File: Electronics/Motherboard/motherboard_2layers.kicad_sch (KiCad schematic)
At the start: 55 parts, among them J1 DX07S024JJ3R1300, J2 Conn_02x10_Odd_Even, M1 AO3400A, M2 AO3400A, M3 AO3400A, U1 AMS1117-3.3, U2 TMC2209_SILENTSTEPSTICK, U3 TMC2209_SILENTSTEPSTICK, U4 TMC2209_SILENTSTEPSTICK, U5 TMC2209_SILENTSTEPSTICK, U6 LM2576HVS-5, U7 STM32G0B1VETx

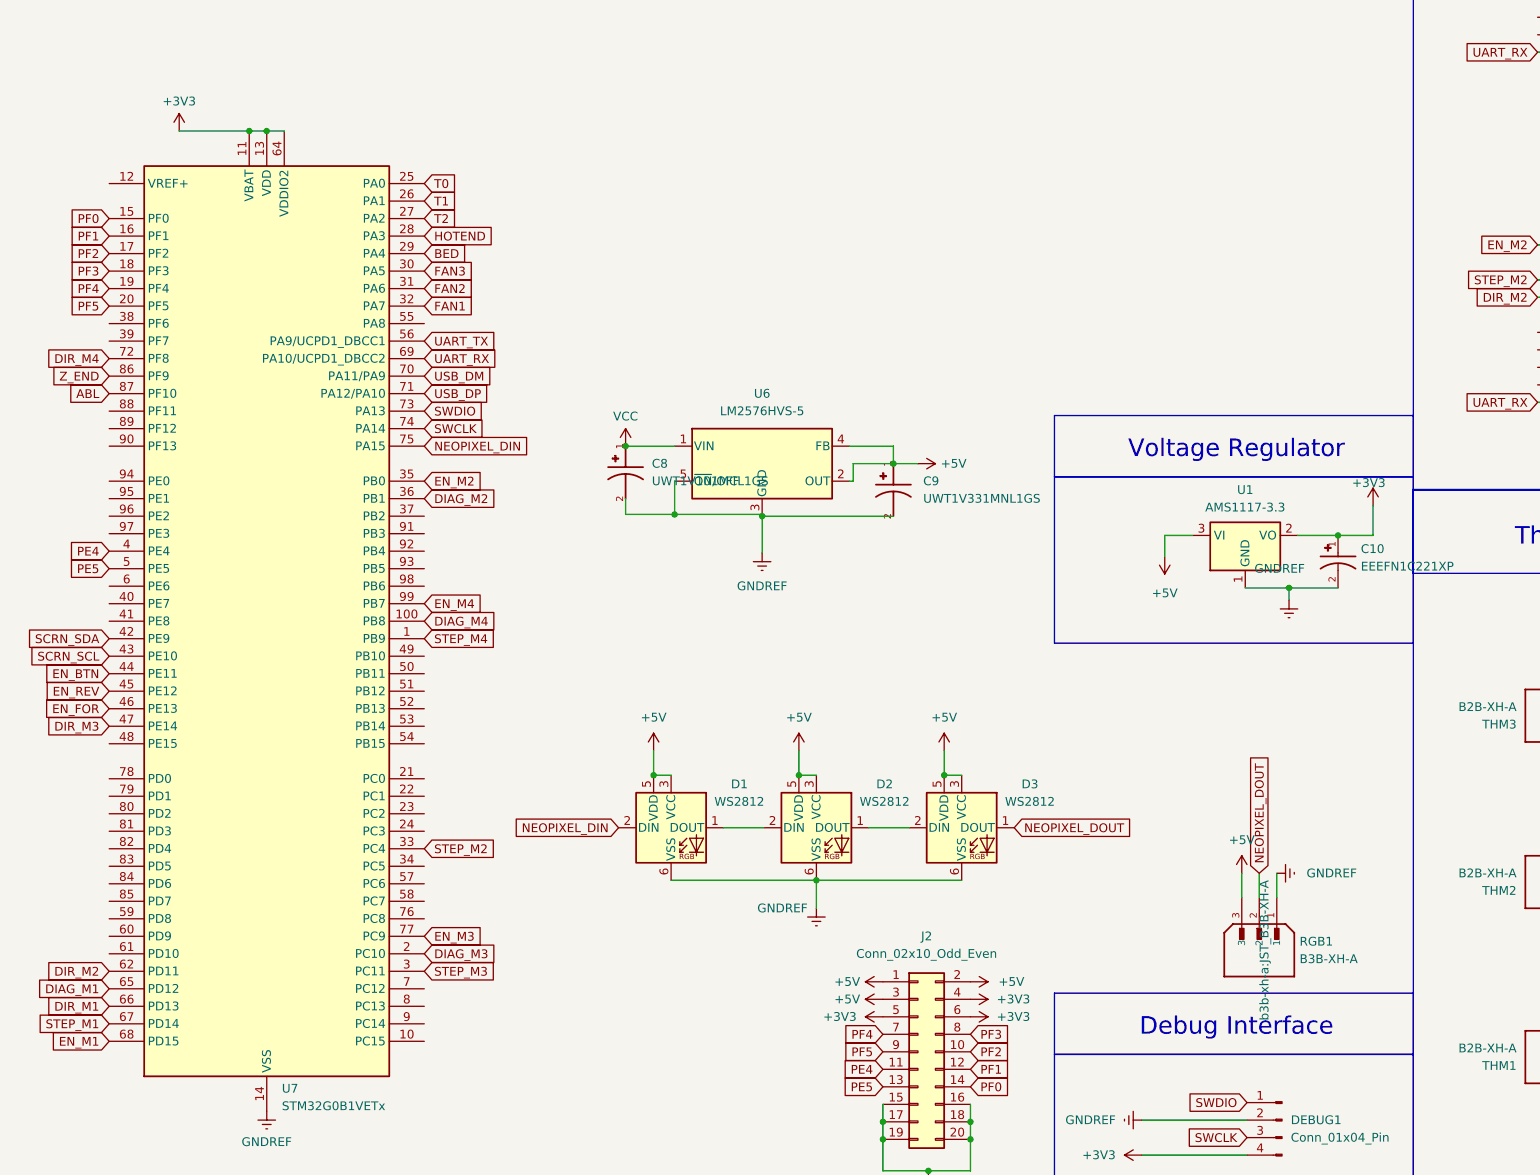
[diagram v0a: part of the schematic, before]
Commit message: yay finished
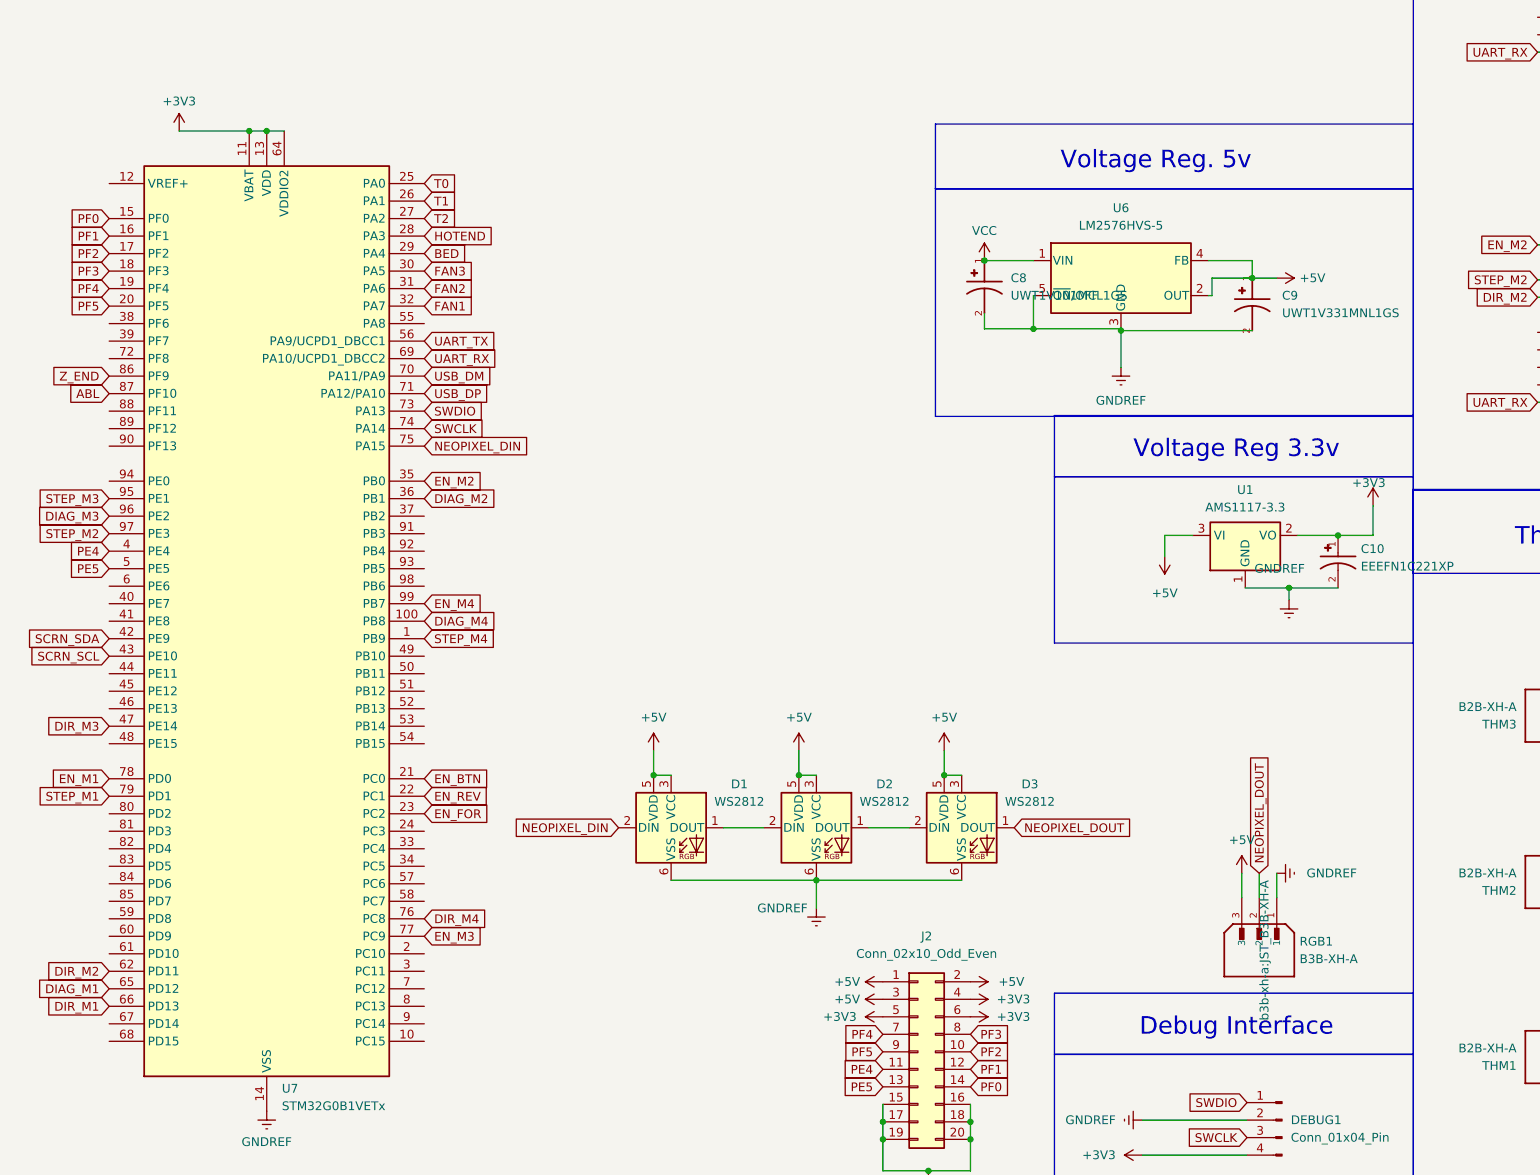
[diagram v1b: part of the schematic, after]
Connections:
- net DIAG_M3: now also U7.96 (PE2); no longer U7.2 (PC10)
- net DIR_M4: now also U7.76 (PC8); no longer U7.72 (PF8)
- net EN_BTN: now also U7.21 (PC0); no longer U7.44 (PE11)
- net EN_FOR: now also U7.23 (PC2); no longer U7.46 (PE13)
- net EN_M1: now also U7.78 (PD0); no longer U7.68 (PD15)
- net EN_REV: now also U7.22 (PC1); no longer U7.45 (PE12)
- net STEP_M1: now also U7.79 (PD1); no longer U7.67 (PD14)
- net STEP_M2: now also U7.97 (PE3); no longer U7.33 (PC4)
- net STEP_M3: now also U7.95 (PE1); no longer U7.3 (PC11)
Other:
- note added: "Voltage Reg 3.3v"
- note added: "Voltage Reg. 5v"
- note removed: "Voltage Regulator"
- moved on the sheet: C8, C9, U6

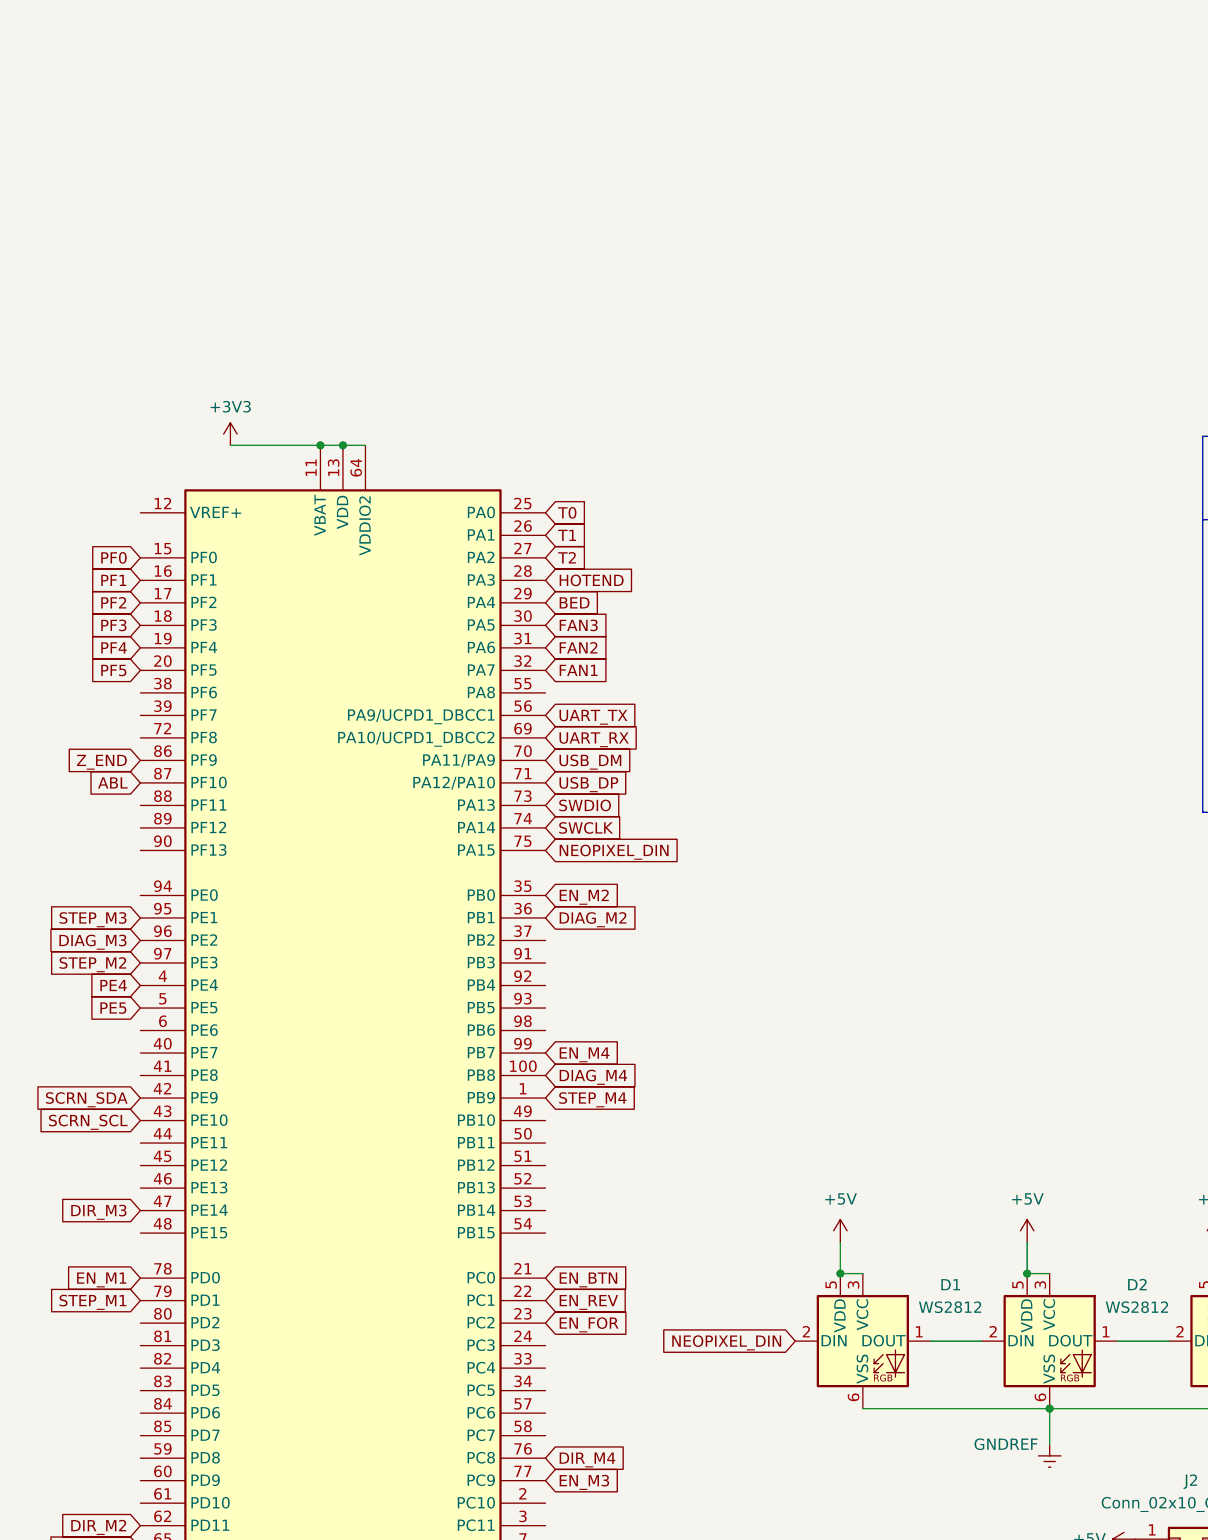
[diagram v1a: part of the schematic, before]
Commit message: updated some files
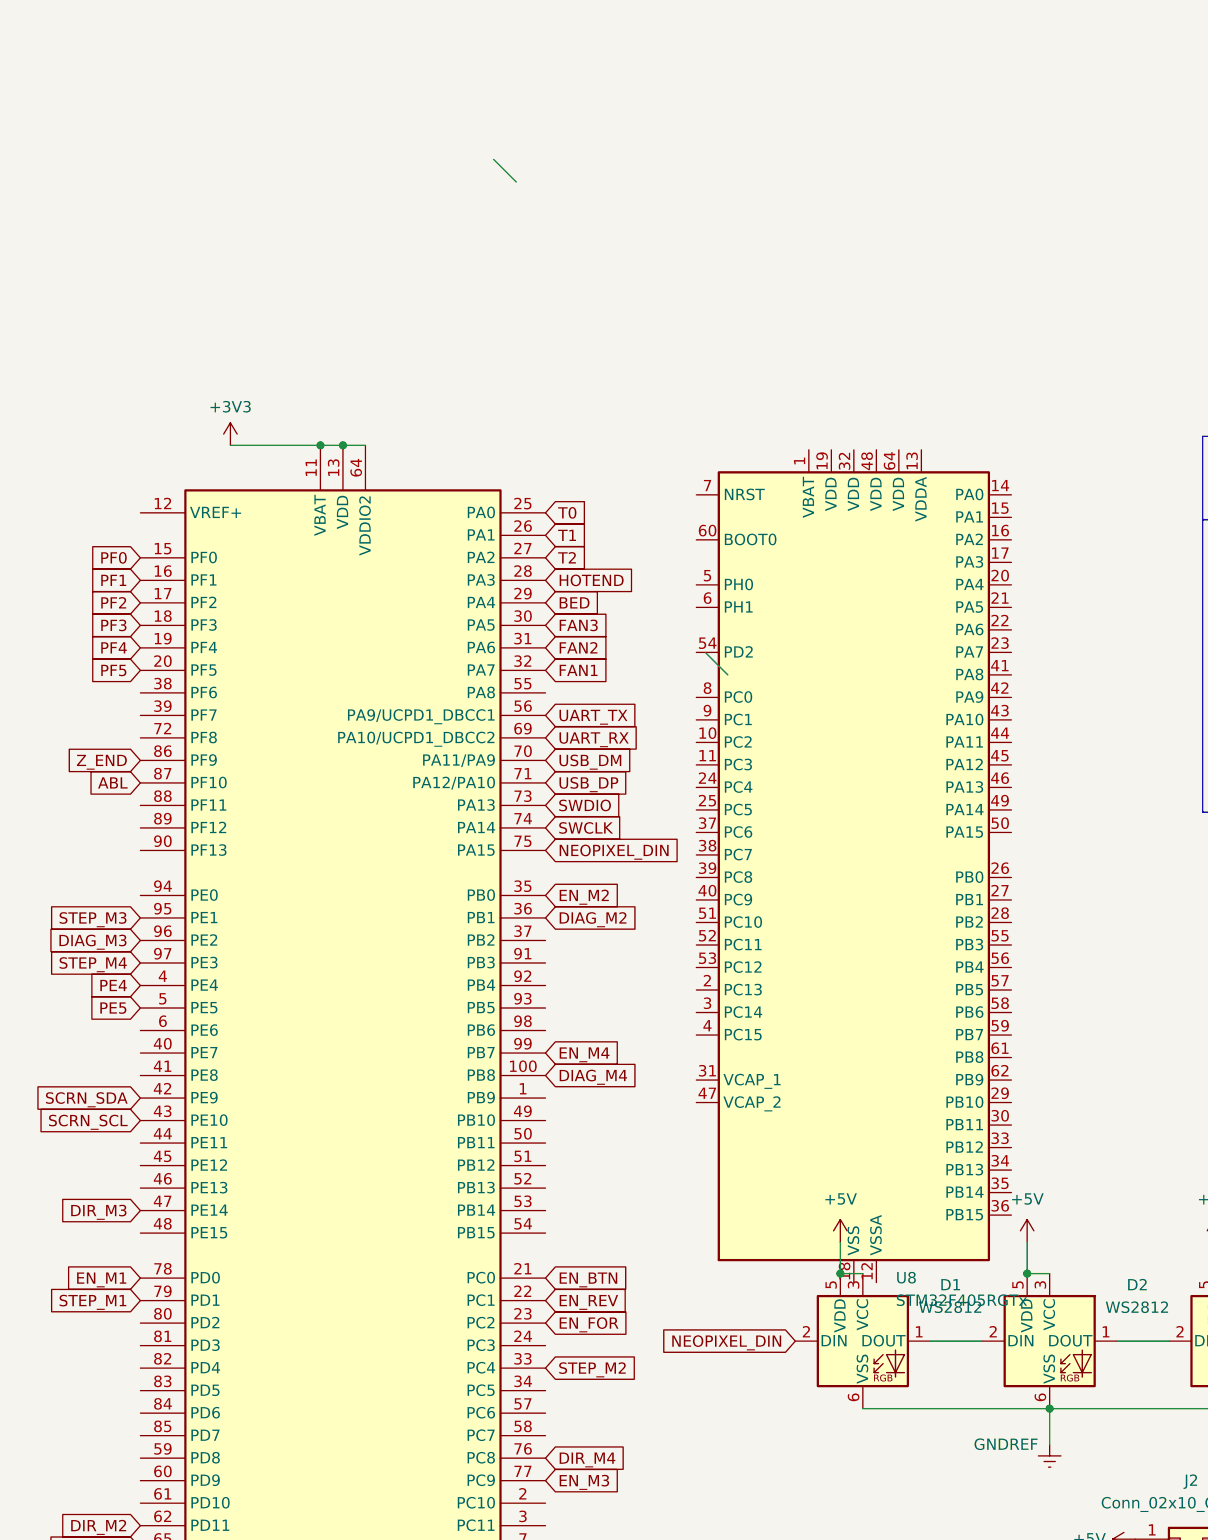
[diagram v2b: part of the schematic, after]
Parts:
- added U8: STM32F405RGTx, Package_QFP:LQFP-64_10x10mm_P0.5mm, symbol MCU_ST_STM32F4:STM32F405RGTx
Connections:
- net STEP_M2: now also U7.33 (PC4); no longer U7.97 (PE3)
- net STEP_M4: now also U7.97 (PE3); no longer U7.1 (PB9)
- new net: U8.18 (VSS), U8.63 (VSS)
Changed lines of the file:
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@@
 		(color 0 0 0 0)
 	)
+	(bus_entry
+		(at 103.124 97.028)
+		(size 2.54 2.54)
+		(stroke
+			(width 0)
+			(type default)
+		)
+	)
+	(bus_entry
+		(at 79.248 41.402)
+		(size 2.54 2.54)
+		(stroke
+			(width 0)
+			(type default)
+		)
+	)
 	(wire
 		(pts
@@
 		)
 	)
+	(global_label "STEP_M4"
+		(shape input)
+		(at 39.37 132.08 180)
+		(fields_autoplaced yes)
+		(effects
+			(font
+				(size 1.27 1.27)
+			)
+			(justify right)
+		)
+		(property "Intersheetrefs" "${INTERSHEET_REFS}"
+			(at 28.1602 132.08 0)
+			(effects
+				(font
+					(size 1.27 1.27)
+				)
+				(justify right)
+				(hide yes)
+			)
+		)
+	)
 	(global_label "ABL"
 		(shape input)
@@
 		)
 	)
-	(global_label "STEP_M4"
-		(shape input)
-		(at 85.09 147.32 0)
-		(fields_autoplaced yes)
-		(effects
-			(font
-				(size 1.27 1.27)
-			)
-			(justify left)
-		)
-		(property "Intersheetrefs" "${INTERSHEET_REFS}"
-			(at 96.2998 147.32 0)
-			(effects
-				(font
-					(size 1.27 1.27)
-				)
-				(justify left)
-				(hide yes)
-			)
-		)
-	)
 	(global_label "UART_TX"
 		(shape input)
@@
 		)
 	)
-	(global_label "STEP_M2"
-		(shape input)
-		(at 39.37 132.08 180)
-		(fields_autoplaced yes)
-		(effects
-			(font
-				(size 1.27 1.27)
-			)
-			(justify right)
-		)
-		(property "Intersheetrefs" "${INTERSHEET_REFS}"
-			(at 28.1602 132.08 0)
-			(effects
-				(font
-					(size 1.27 1.27)
-				)
-				(justify right)
-				(hide yes)
-			)
-		)
-	)
 	(global_label "EN_M3"
 		(shape input)
@@
 		)
 	)
+	(global_label "STEP_M2"
+		(shape input)
+		(at 85.09 177.8 0)
+		(fields_autoplaced yes)
+		(effects
+			(font
+				(size 1.27 1.27)
+			)
+			(justify left)
+		)
+		(property "Intersheetrefs" "${INTERSHEET_REFS}"
+			(at 96.2998 177.8 0)
+			(effects
+				(font
+					(size 1.27 1.27)
+				)
+				(justify left)
+				(hide yes)
+			)
+		)
+	)
 	(global_label "UART_TX"
 		(shape input)
@@
 					(unit 1)
 				)
+			)
+		)
+	)
+	(symbol
+		(lib_id "MCU_ST_STM32F4:STM32F405RGTx")
+		(at 119.888 122.428 0)
+		(unit 1)
+		(exclude_from_sim no)
+		(in_bom yes)
+		(on_board yes)
+		(dnp no)
+		(fields_autoplaced yes)
+		(property "Reference" "U8"
+			(at 124.6221 167.64 0)
+			(effects
+				(font
+					(size 1.27 1.27)
+				)
+				(justify left)
+			)
+		)
+		(property "Value" "STM32F405RGTx"
+			(at 124.6221 170.18 0)
+			(effects
+				(font
+					(size 1.27 1.27)
+				)
+				(justify left)
+			)
+		)
+		(property "Footprint" "Package_QFP:LQFP-64_10x10mm_P0.5mm"
+			(at 104.648 165.608 0)
+			(effects
+				(font
+					(size 1.27 1.27)
+				)
+				(justify right)
+				(hide yes)
+			)
+		)
+		(property "Datasheet" "https://www.st.com/resource/en/datasheet/stm32f405rg.pdf"
+			(at 119.888 122.428 0)
+			(effects
+				(font
+					(size 1.27 1.27)
+				)
+				(hide yes)
+			)
+		)
+		(property "Description" "STMicroelectronics Arm Cortex-M4 MCU, 1024KB flash, 192KB RAM, 168 MHz, 1.8-3.6V, 51 GPIO, LQFP64"
+			(at 119.888 122.428 0)
+			(effects
+				(font
+					(size 1.27 1.27)
+				)
+				(hide yes)
+			)
+		)
+		(pin "63"
+		)
+		(pin "7"
+		)
+		(pin "50"
+		)
+		(pin "31"
+		)
+		(pin "33"
+		)
+		(pin "12"
+		)
+		(pin "34"
+		)
+		(pin "39"
+		)
+		(pin "44"
+		)
+		(pin "46"
+		)
+		(pin "60"
+		)
+		(pin "20"
+		)
+		(pin "36"
+		)
+		(pin "55"
+		)
+		(pin "15"
+		)
+		(pin "18"
+		)
+		(pin "37"
+		)
+		(pin "58"
+		)
+		(pin "2"
+		)
+		(pin "47"
+		)
+		(pin "5"
+		)
+		(pin "54"
+		)
+		(pin "62"
+		)
+		(pin "13"
+		)
+		(pin "53"
+		)
+		(pin "56"
+		)
+		(pin "27"
+		)
+		(pin "42"
+		)
+		(pin "59"
+		)
+		(pin "40"
+		)
+		(pin "64"
+		)
+		(pin "19"
+		)
+		(pin "48"
+		)
+		(pin "23"
+		)
+		(pin "32"
+		)
+		(pin "22"
+		)
+		(pin "41"
+		)
+		(pin "17"
+		)
+		(pin "49"
+		)
+		(pin "30"
+		)
+		(pin "10"
+		)
+		(pin "51"
+		)
+		(pin "43"
+		)
+		(pin "57"
+		)
+		(pin "6"
+		)
+		(pin "61"
+		)
+		(pin "26"
+		)
+		(pin "1"
+		)
+		(pin "11"
+		)
+		(pin "14"
+		)
+		(pin "16"
+		)
+		(pin "21"
+		)
+		(pin "25"
+		)
+		(pin "28"
+		)
+		(pin "29"
+		)
+		(pin "3"
+		)
+		(pin "38"
+		)
+		(pin "4"
+		)
+		(pin "45"
+		)
+		(pin "52"
+		)
+		(pin "35"
+		)
+		(pin "24"
+		)
+		(pin "9"
+		)
+		(pin "8"
+		)
+		(instances
+			(project ""
+				(path "/9290e430-09f5-4a3f-8744-4071dceedc2e"
+					(reference "U8")
+					(unit 1)
+				)
